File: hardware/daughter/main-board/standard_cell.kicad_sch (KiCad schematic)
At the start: 13 parts, among them J5 Conn_01x02_Pin, U10 TL071, U11 CD22M3494MQZ, U12 CD22M3494MQZ, U7 TL071, U8 AD5263BRUZ200, U9 AD5263BRUZ200

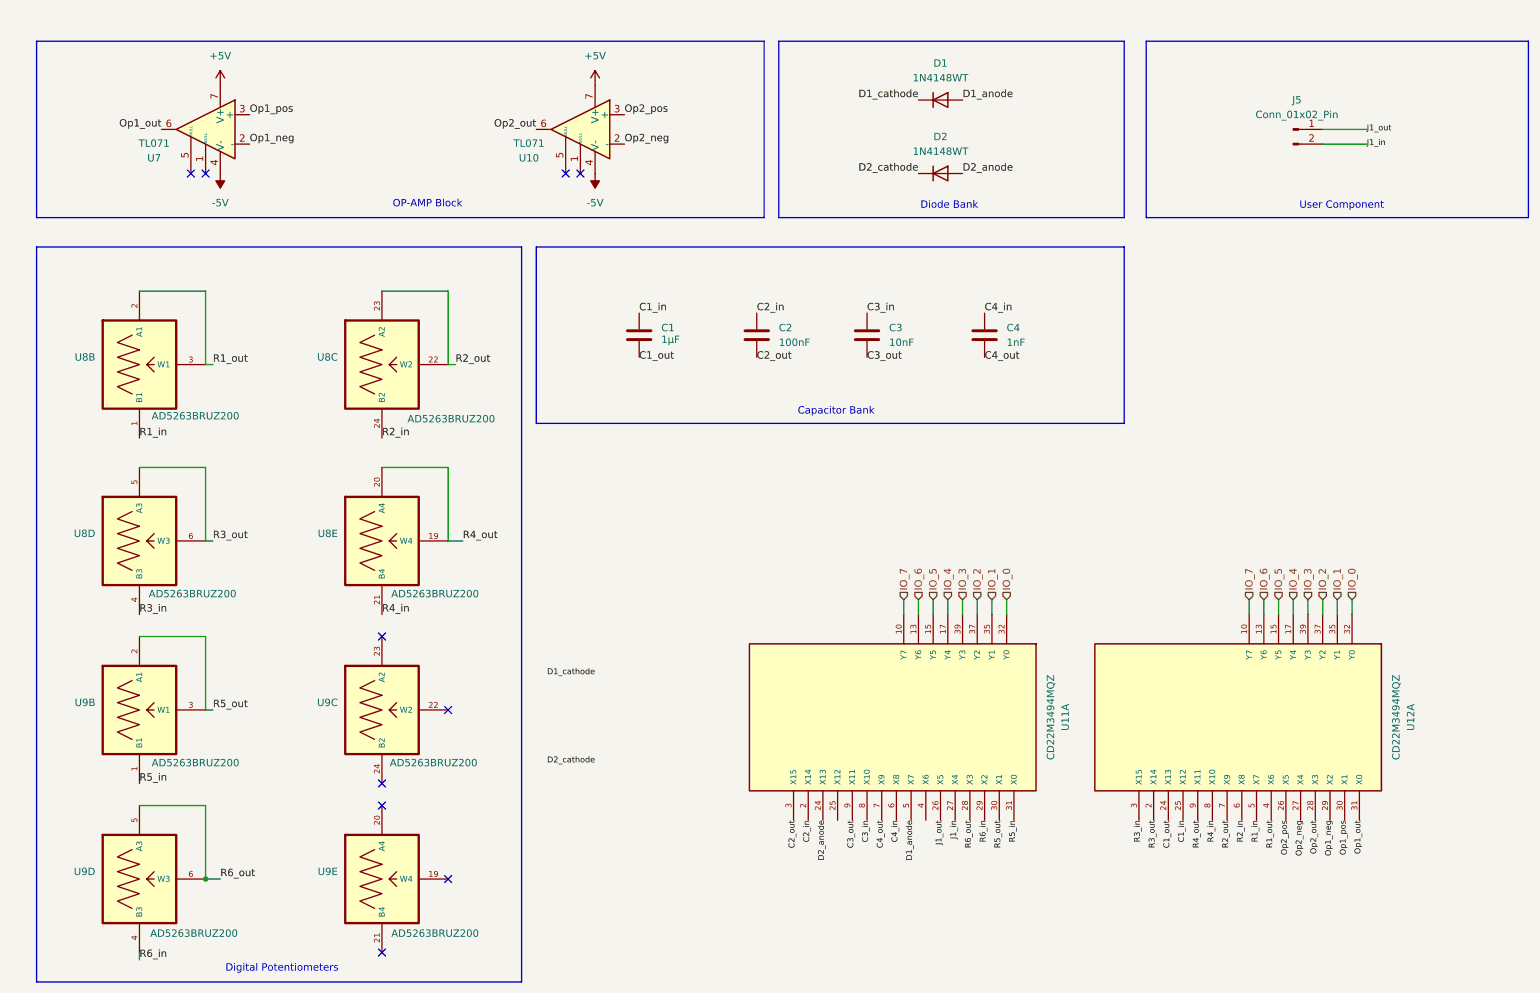
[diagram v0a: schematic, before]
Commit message: Updated daughter board schematic
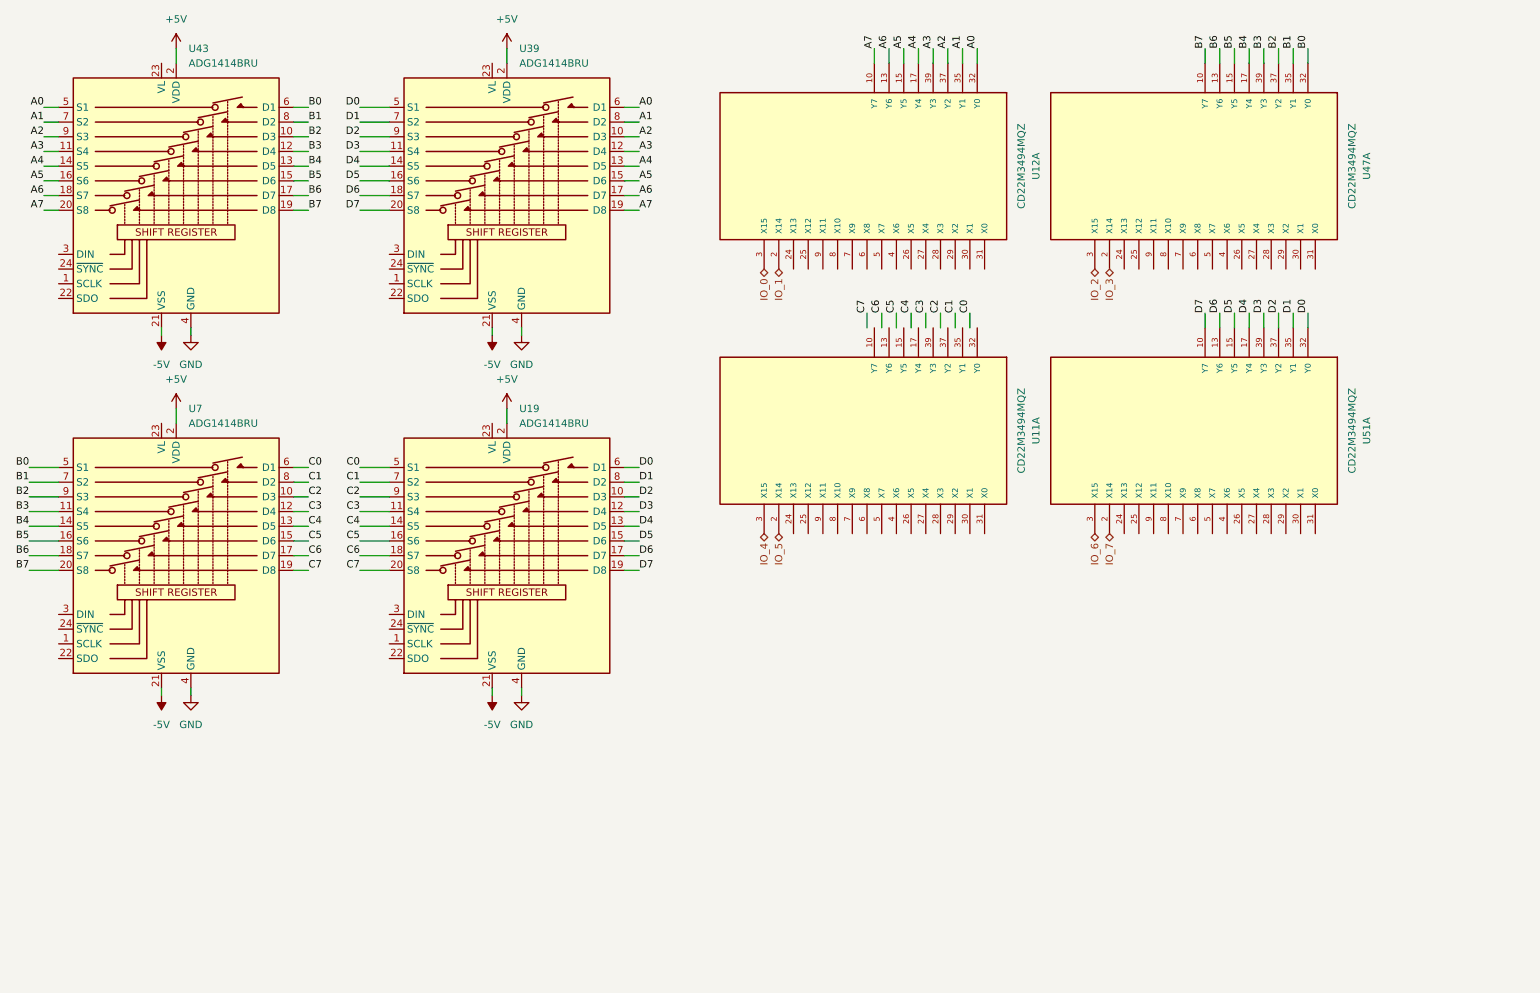
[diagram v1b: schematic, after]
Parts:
- removed C1: 1µF, Capacitor_SMD:C_0603_1608Metric_Pad1.08x0.95mm_HandSolder, symbol Device:C
- removed C2: 100nF, Capacitor_SMD:C_0603_1608Metric_Pad1.08x0.95mm_HandSolder, symbol Device:C
- removed C3: 10nF, Capacitor_SMD:C_0603_1608Metric_Pad1.08x0.95mm_HandSolder, symbol Device:C
- removed C4: 1nF, Capacitor_SMD:C_0603_1608Metric_Pad1.08x0.95mm_HandSolder, symbol Device:C
- removed D1, D2: 1N4148WT, Diode_SMD:D_SOD-123, symbol Diode:1N4148WT
- removed J5: Conn_01x02_Pin, Connector_PinSocket_2.54mm:PinSocket_1x02_P2.54mm_Vertical, symbol Connector:Conn_01x02_Pin
- removed U10, U7: TL071, Package_SO:SOIC-8_3.9x4.9mm_P1.27mm, symbol Amplifier_Operational:TL071
- removed U8, U9: AD5263BRUZ200, SeniorDesignFP:SOP65P640X120-24N, symbol SeniorDesign:AD5263BRUZ200
- added U19, U39, U43, U7: ADG1414BRU, Package_SO:TSSOP-24_4.4x7.8mm_P0.65mm, symbol Analog_Switch:ADG1414BRU
- added U47, U51: CD22M3494MQZ, SeniorDesignFP:PLCC44_16P66X16P66_INR-M, symbol SeniorDesign:CD22M3494MQZ
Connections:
- net C2_in is gone; now on net IO_5: U11.2 (X14)
- net C2_out is gone; now on net IO_4: U11.3 (X15)
- net R3_in is gone; now on net IO_0: U12.3 (X15)
- net R3_out is gone; now on net IO_1: U12.2 (X14)
- net +5V: now also U19.2 (VDD), U39.2 (VDD), U43.2 (VDD), U7.2 (VDD)
- net -5V: now also U19.21 (VSS), U39.21 (VSS), U43.21 (VSS), U7.21 (VSS)
- net IO_0: no longer U11.32 (Y0), U12.32 (Y0)
- net IO_1: no longer U11.35 (Y1), U12.35 (Y1)
- net IO_2: now also U47.3 (X15); no longer U11.37 (Y2), U12.37 (Y2)
- net IO_3: now also U47.2 (X14); no longer U11.39 (Y3), U12.39 (Y3)
- net IO_4: no longer U11.17 (Y4), U12.17 (Y4)
- net IO_5: no longer U11.15 (Y5), U12.15 (Y5)
- net IO_6: now also U51.3 (X15); no longer U11.13 (Y6), U12.13 (Y6)
- net IO_7: now also U51.2 (X14); no longer U11.10 (Y7), U12.10 (Y7)
- net C1_in: no longer names the net of U12.25 (X12)
- net C1_out: no longer names the net of U12.24 (X13)
- net C3_in: no longer names the net of U11.8 (X10)
- net C3_out: no longer names the net of U11.9 (X11)
- net C4_in: no longer names the net of U11.6 (X8)
- net C4_out: no longer names the net of U11.7 (X9)
- net D1_anode: no longer names the net of U11.5 (X7)
- net D2_anode: no longer names the net of U11.24 (X13)
- net J1_in: no longer names the net of U11.27 (X4)
- net J1_out: no longer names the net of U11.26 (X5)
- net Op1_neg: no longer names the net of U12.29 (X2)
- net Op1_out: no longer names the net of U12.31 (X0)
- net Op1_pos: no longer names the net of U12.30 (X1)
- net Op2_neg: no longer names the net of U12.27 (X4)
- net Op2_out: no longer names the net of U12.28 (X3)
- net Op2_pos: no longer names the net of U12.26 (X5)
- net R1_in: no longer names the net of U12.5 (X7)
- net R1_out: no longer names the net of U12.4 (X6)
- net R2_in: no longer names the net of U12.6 (X8)
- net R2_out: no longer names the net of U12.7 (X9)
- net R4_in: no longer names the net of U12.8 (X10)
- net R4_out: no longer names the net of U12.9 (X11)
- net R5_in: no longer names the net of U11.31 (X0)
- net R5_out: no longer names the net of U11.30 (X1)
- net R6_in: no longer names the net of U11.29 (X2)
- net R6_out: no longer names the net of U11.28 (X3)
- new net A0: U12.32 (Y0), U39.6 (D1), U43.5 (S1)
- new net A1: U12.35 (Y1), U39.8 (D2), U43.7 (S2)
- new net A2: U12.37 (Y2), U39.10 (D3), U43.9 (S3)
- new net A3: U12.39 (Y3), U39.12 (D4), U43.11 (S4)
- new net A4: U12.17 (Y4), U39.13 (D5), U43.14 (S5)
- new net A5: U12.15 (Y5), U39.15 (D6), U43.16 (S6)
- new net A6: U12.13 (Y6), U39.17 (D7), U43.18 (S7)
- new net A7: U12.10 (Y7), U39.19 (D8), U43.20 (S8)
- new net B0: U43.6 (D1), U47.32 (Y0), U7.5 (S1)
- new net B1: U43.8 (D2), U47.35 (Y1), U7.7 (S2)
- new net B2: U43.10 (D3), U47.37 (Y2), U7.9 (S3)
- new net B3: U43.12 (D4), U47.39 (Y3), U7.11 (S4)
- new net B4: U43.13 (D5), U47.17 (Y4), U7.14 (S5)
- new net B5: U43.15 (D6), U47.15 (Y5), U7.16 (S6)
- new net B6: U43.17 (D7), U47.13 (Y6), U7.18 (S7)
- new net B7: U43.19 (D8), U47.10 (Y7), U7.20 (S8)
- new net C0: U19.5 (S1), U7.6 (D1)
- new net C1: U19.7 (S2), U7.8 (D2)
- new net C2: U19.9 (S3), U7.10 (D3)
- new net C3: U19.11 (S4), U7.12 (D4)
- new net C4: U19.14 (S5), U7.13 (D5)
- new net C5: U19.16 (S6), U7.15 (D6)
- new net C6: U19.18 (S7), U7.17 (D7)
- new net C7: U19.20 (S8), U7.19 (D8)
- new net D0: U19.6 (D1), U39.5 (S1), U51.32 (Y0)
- new net D1: U19.8 (D2), U39.7 (S2), U51.35 (Y1)
- new net D2: U19.10 (D3), U39.9 (S3), U51.37 (Y2)
- new net D3: U19.12 (D4), U39.11 (S4), U51.39 (Y3)
- new net D4: U19.13 (D5), U39.14 (S5), U51.17 (Y4)
- new net D5: U19.15 (D6), U39.16 (S6), U51.15 (Y5)
- new net D6: U19.17 (D7), U39.18 (S7), U51.13 (Y6)
- new net D7: U19.19 (D8), U39.20 (S8), U51.10 (Y7)
- new net GND: U19.4 (GND), U39.4 (GND), U43.4 (GND), U7.4 (GND)
- no-connect marks 10 -> 0
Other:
- note removed: "Capacitor Bank"
- note removed: "Digital Potentiometers"
- note removed: "Diode Bank"
- note removed: "OP-AMP Block"
- note removed: "User Component"
- moved on the sheet: U12A
